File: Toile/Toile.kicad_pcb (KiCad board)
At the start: 2 copper layers, 170.2 x 99.1 mm, 2 parts

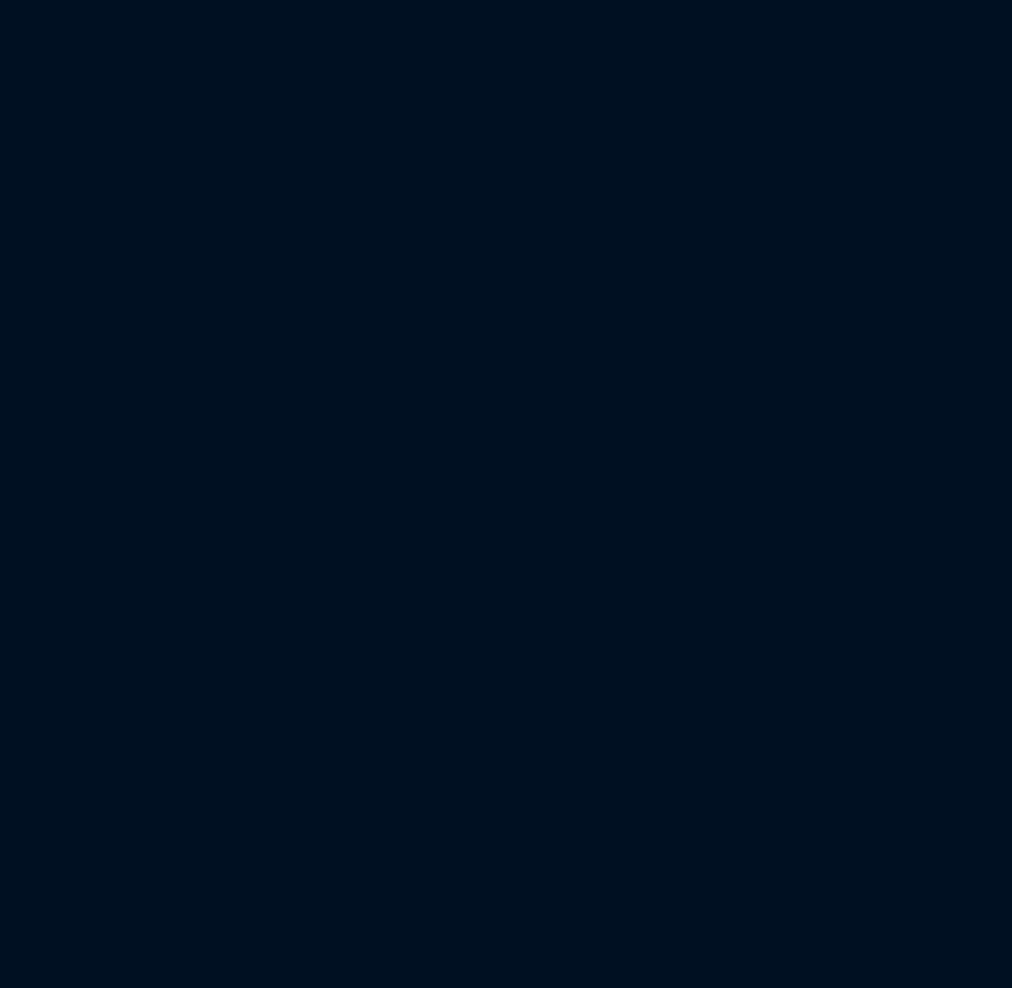
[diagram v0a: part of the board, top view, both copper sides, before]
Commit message: Cours du 22.06.2020
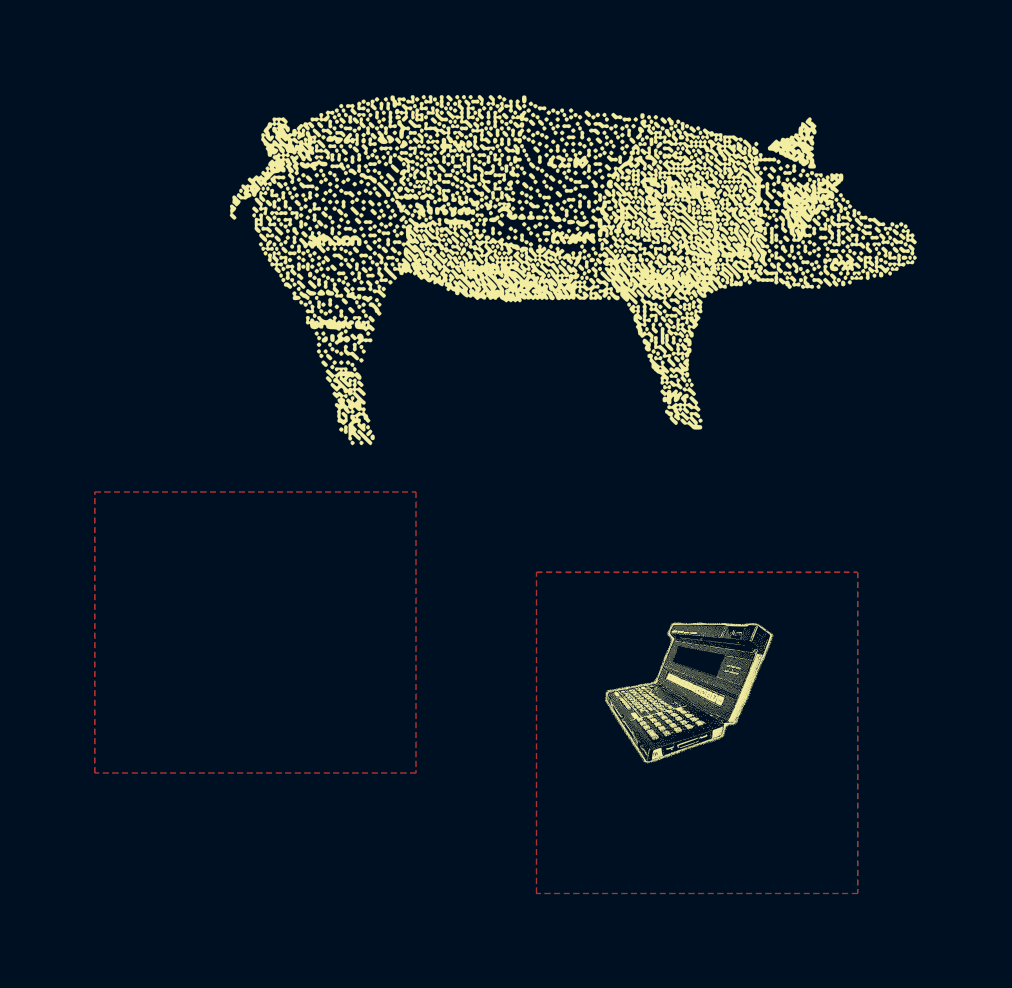
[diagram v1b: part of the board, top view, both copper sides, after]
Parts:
- added G***: LOGO, Alexx:PB_1000_screen_soldermask, F.Cu at (167.6, 109.2)
- added G***: LOGO, Alexx:PB_1000_cutout_silk, F.Cu at (167.6, 109.2)
- added G***: LOGO, CoursPCB:porc_silkscreen, F.Cu at (160.0, 81.3)
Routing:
- added copper zone on F.Cu, net (none)
